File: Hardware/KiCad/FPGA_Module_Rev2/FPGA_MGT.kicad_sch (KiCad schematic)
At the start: 2 parts, among them U1 IC FPGA XC7A50T-2CSG325C

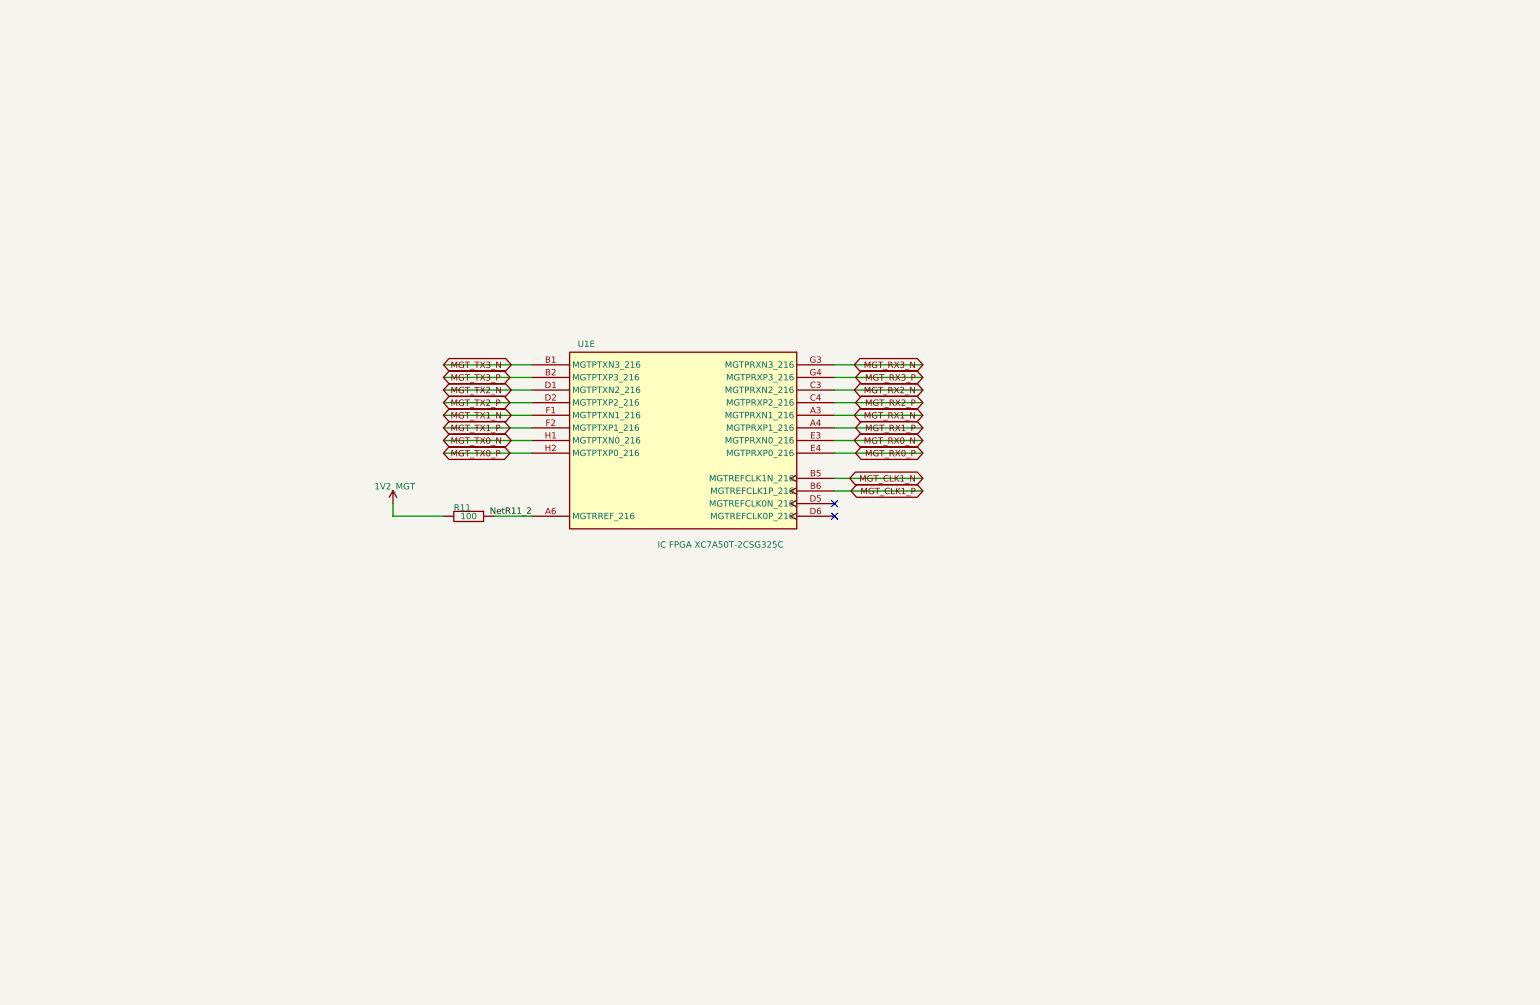
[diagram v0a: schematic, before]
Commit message: Adding the KiCad Design for the FPGA Module Board with no DRC errors
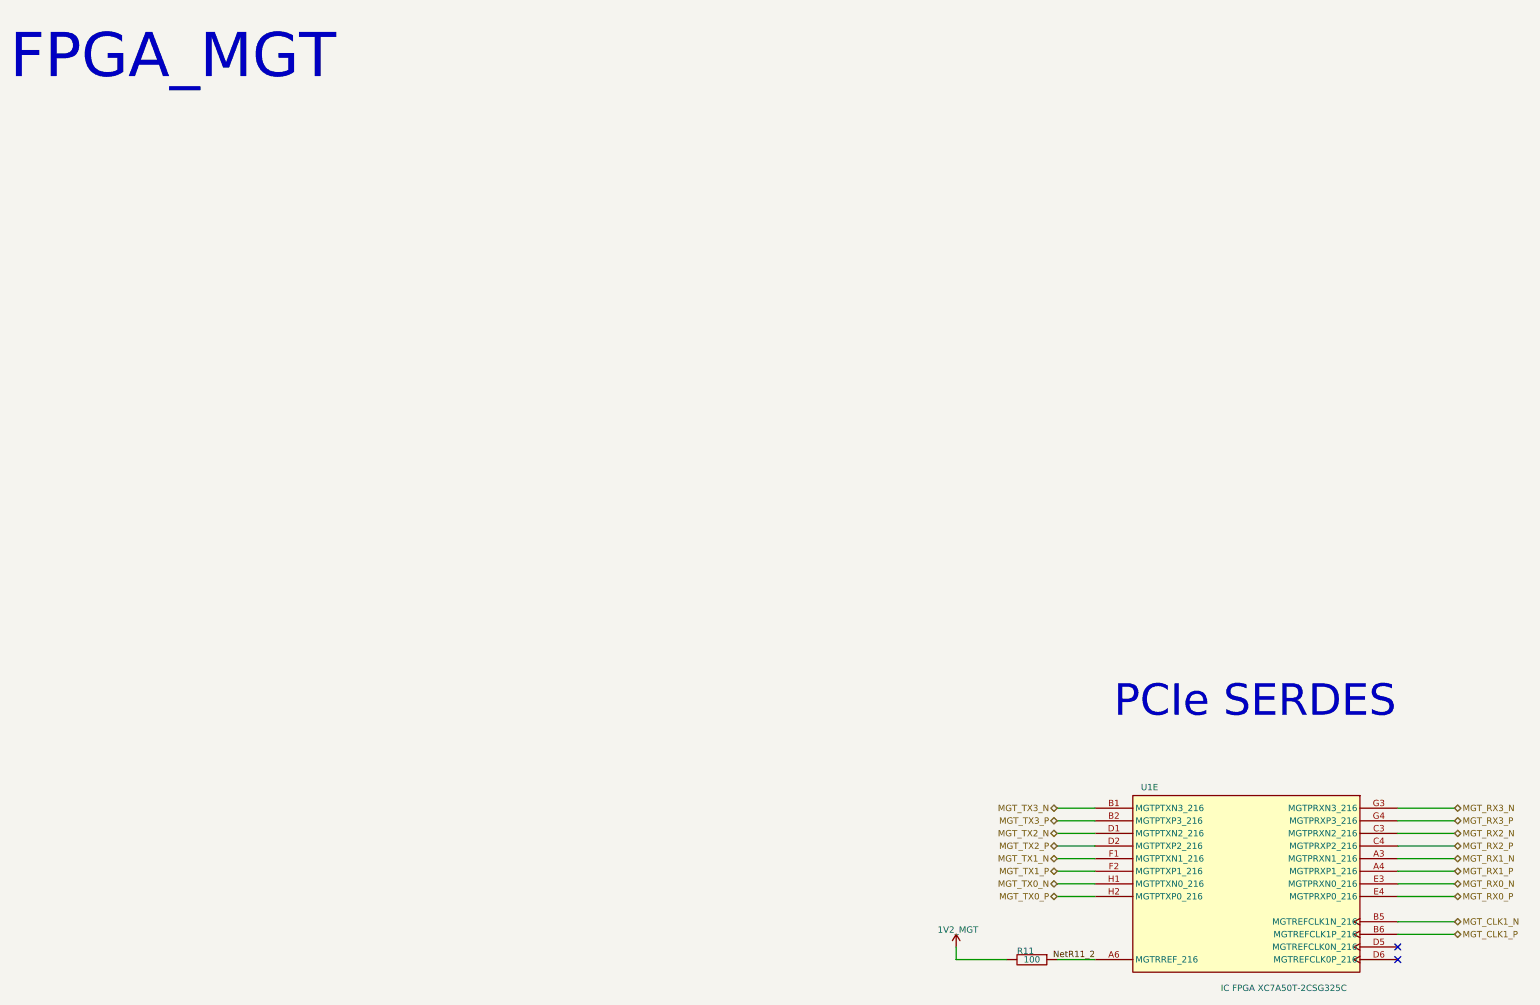
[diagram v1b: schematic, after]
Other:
- note added: "FPGA_MGT"
- note added: "PCIe SERDES"
- moved on the sheet: R11, U1E
